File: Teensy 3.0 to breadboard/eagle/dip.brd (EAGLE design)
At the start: 63.2 x 20.3 mm, 9 parts

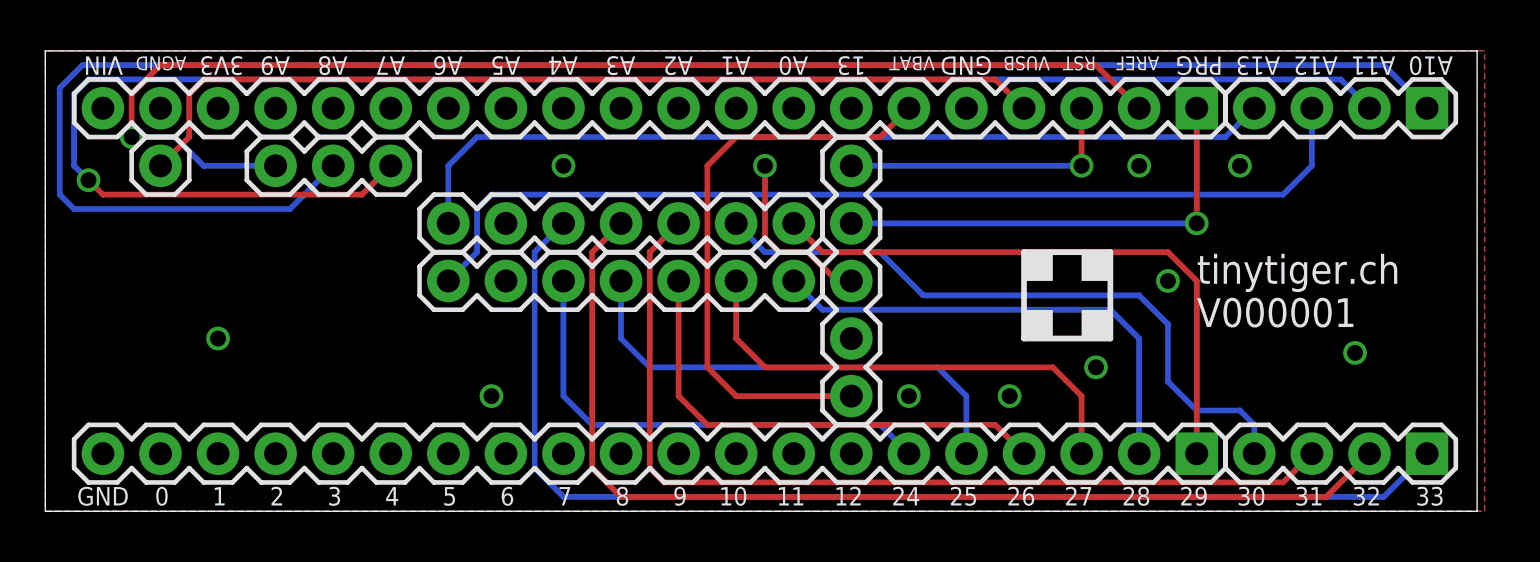
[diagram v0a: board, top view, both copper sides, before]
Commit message: Version 3 final
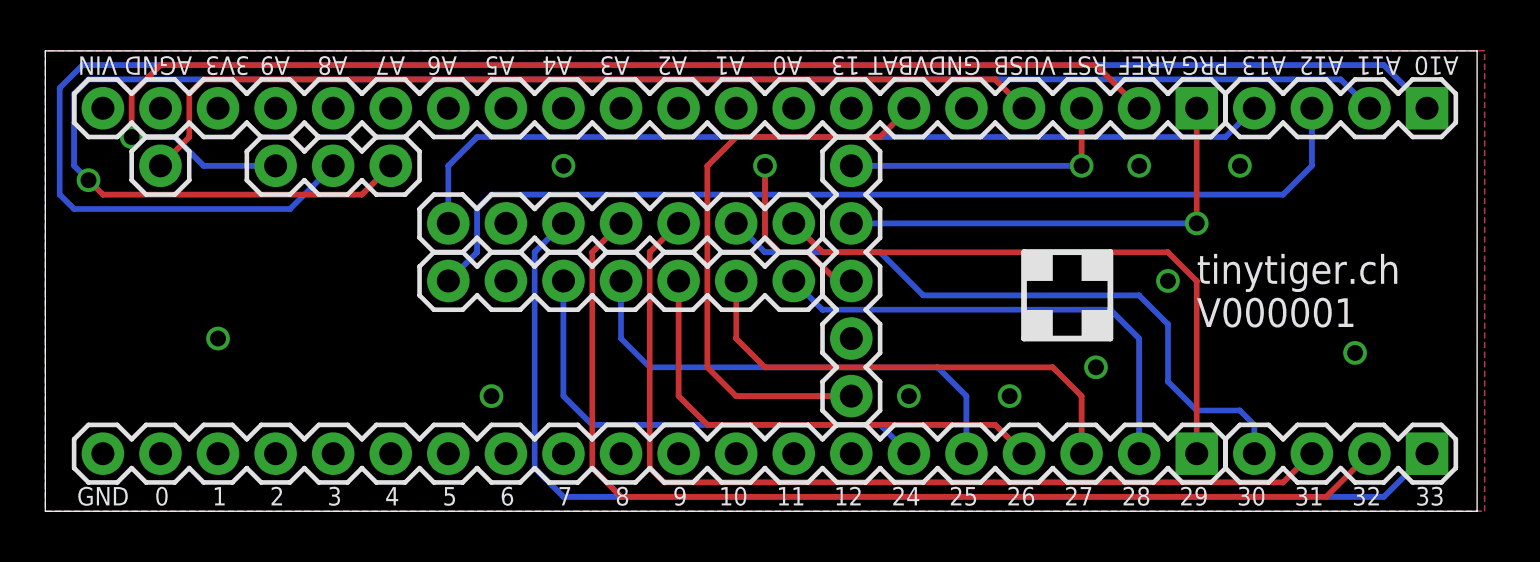
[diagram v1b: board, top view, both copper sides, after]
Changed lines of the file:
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@@
 <setting verticaltext="up"/>
 </settings>
-<grid distance="25" unitdist="mil" unit="mm" style="lines" multiple="1" display="no" altdistance="0.025" altunitdist="inch" altunit="inch"/>
+<grid distance="10" unitdist="mil" unit="mil" style="lines" multiple="1" display="no" altdistance="0.025" altunitdist="inch" altunit="inch"/>
 <layers>
 <layer number="1" name="Top" color="4" fill="1" visible="yes" active="yes"/>
@@
 <text x="57.658" y="0.254" size="0.8128" layer="25">32</text>
 <text x="60.452" y="0.254" size="0.8128" layer="25">33</text>
-<text x="3.429" y="20.066" size="0.8128" layer="25" rot="SR180">VIN</text>
-<text x="6.223" y="20.066" size="0.6096" layer="25" rot="SR180">AGND</text>
-<text x="8.763" y="20.066" size="0.8128" layer="25" rot="SR180">3V3</text>
+<text x="3.175" y="20.066" size="0.8128" layer="25" rot="SR180">VIN</text>
+<text x="6.477" y="20.066" size="0.8128" layer="25" rot="SR180">AGND</text>
+<text x="9.017" y="20.066" size="0.8128" layer="25" rot="SR180">3V3</text>
 <text x="10.795" y="20.066" size="0.8128" layer="25" rot="SR180">A9</text>
 <text x="13.335" y="20.066" size="0.8128" layer="25" rot="SR180">A8</text>
 <text x="15.875" y="20.066" size="0.8128" layer="25" rot="SR180">A7</text>
-<text x="18.415" y="20.066" size="0.8128" layer="25" rot="SR180">A6</text>
-<text x="20.955" y="20.066" size="0.8128" layer="25" rot="SR180">A5</text>
-<text x="23.495" y="20.066" size="0.8128" layer="25" rot="SR180">A4</text>
-<text x="26.035" y="20.066" size="0.8128" layer="25" rot="SR180">A3</text>
-<text x="28.575" y="20.066" size="0.8128" layer="25" rot="SR180">A2</text>
-<text x="31.115" y="20.066" size="0.8128" layer="25" rot="SR180">A1</text>
-<text x="33.655" y="20.066" size="0.8128" layer="25" rot="SR180">A0</text>
-<text x="36.195" y="20.066" size="0.8128" layer="25" rot="SR180">13</text>
-<text x="39.243" y="20.066" size="0.6096" layer="25" rot="SR180">VBAT</text>
-<text x="41.783" y="20.066" size="0.8128" layer="25" rot="SR180">GND</text>
-<text x="44.323" y="20.066" size="0.6096" layer="25" rot="SR180">VUSB</text>
-<text x="46.355" y="20.066" size="0.6096" layer="25" rot="SR180">RST</text>
-<text x="49.149" y="20.066" size="0.6096" layer="25" rot="SR180">AREF</text>
-<text x="51.943" y="20.066" size="0.8128" layer="25" rot="SR180">PRG</text>
-<text x="54.483" y="20.066" size="0.8128" layer="25" rot="SR180">A13</text>
-<text x="57.023" y="20.066" size="0.8128" layer="25" rot="SR180">A12</text>
-<text x="59.563" y="20.066" size="0.8128" layer="25" rot="SR180">A11</text>
-<text x="62.103" y="20.066" size="0.8128" layer="25" rot="SR180">A10</text>
+<text x="18.161" y="20.066" size="0.8128" layer="25" rot="SR180">A6</text>
+<text x="20.701" y="20.066" size="0.8128" layer="25" rot="SR180">A5</text>
+<text x="23.241" y="20.066" size="0.8128" layer="25" rot="SR180">A4</text>
+<text x="25.781" y="20.066" size="0.8128" layer="25" rot="SR180">A3</text>
+<text x="28.321" y="20.066" size="0.8128" layer="25" rot="SR180">A2</text>
+<text x="30.861" y="20.066" size="0.8128" layer="25" rot="SR180">A1</text>
+<text x="33.401" y="20.066" size="0.8128" layer="25" rot="SR180">A0</text>
+<text x="35.941" y="20.066" size="0.8128" layer="25" rot="SR180">13</text>
+<text x="38.989" y="20.066" size="0.8128" layer="25" rot="SR180">VBAT</text>
+<text x="41.275" y="20.066" size="0.8128" layer="25" rot="SR180">GND</text>
+<text x="44.577" y="20.066" size="0.8128" layer="25" rot="SR180">VUSB</text>
+<text x="46.863" y="20.066" size="0.8128" layer="25" rot="SR180">RST</text>
+<text x="49.911" y="20.066" size="0.8128" layer="25" rot="SR180">AREF</text>
+<text x="52.197" y="20.066" size="0.8128" layer="25" rot="SR180">PRG</text>
+<text x="54.737" y="20.066" size="0.8128" layer="25" rot="SR180">A13</text>
+<text x="57.277" y="20.066" size="0.8128" layer="25" rot="SR180">A12</text>
+<text x="59.817" y="20.066" size="0.8128" layer="25" rot="SR180">A11</text>
+<text x="62.357" y="20.066" size="0.8128" layer="25" rot="SR180">A10</text>
 <text x="50.8" y="8.128" size="1.27" layer="25">tinytiger.ch
 V000001</text>
